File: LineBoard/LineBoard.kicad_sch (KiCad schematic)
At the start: 0 parts

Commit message: サイドセンサプルアップ追加
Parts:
- added C1: C_Small, Capacitor_SMD:C_0603_1608Metric_Pad1.08x0.95mm_HandSolder, symbol Device:C_Small
- added D1: IR17-21C/TR8, LED_SMD:LED_0805_2012Metric, symbol Device:LED
- added D2: IR17-21C/TR8, Diode_SMD:D_0805_2012Metric_Pad1.15x1.40mm_HandSolder, symbol Device:LED_Small
- added IC1: S7136, S7136:DIP575W60P254L560H210Q4N, symbol 0_Aslan2:S7136
- added J1: side_l, Connector_JST:JST_PH_B3B-PH-K_1x03_P2.00mm_Vertical, symbol Connector_Generic:Conn_01x03
- added Q1: PT17-21B/L41/TR8, Diode_SMD:D_0805_2012Metric, symbol Device:Q_Photo_NPN
- added R1: 180, Resistor_SMD:R_0603_1608Metric, symbol Device:R
- added R2: 10k, Resistor_SMD:R_0603_1608Metric, symbol Device:R
- added R3: 420, Resistor_SMD:R_0603_1608Metric_Pad0.98x0.95mm_HandSolder, symbol Device:R_Small
- added R4: 5.6k, Resistor_SMD:R_0402_1005Metric, symbol Device:R_Small
- added R5: 10k, Resistor_SMD:R_0402_1005Metric, symbol Device:R_Small
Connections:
- new net: D2.2 (A), R3.1
- new net: IC1.3 (VOUT), J1.3 (Pin_3), R4.2, R5.1
- new net: D2.1 (K), IC1.1 (CATHODE_(LED))
- new net: D1.2 (A), R1.2
- new net +3V3: Q1.1 (C)
- new net +5V: C1.1, IC1.2 (VCC), J1.2 (Pin_2), R1.1, R3.2, R4.1
- new net GND: C1.2, D1.1 (K), IC1.4 (GND), J1.1 (Pin_1), R2.2, R5.2
- new net VOUT: Q1.2 (E), R2.1
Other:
- note added: "IR17-21C/TR8 (5V) + PT17-21B/L41/TR8 (3.3V) reflective photo-reflector R1=180R sets IF≈21mA. R2=10k pull-up (tune experimentally by reflectance)."

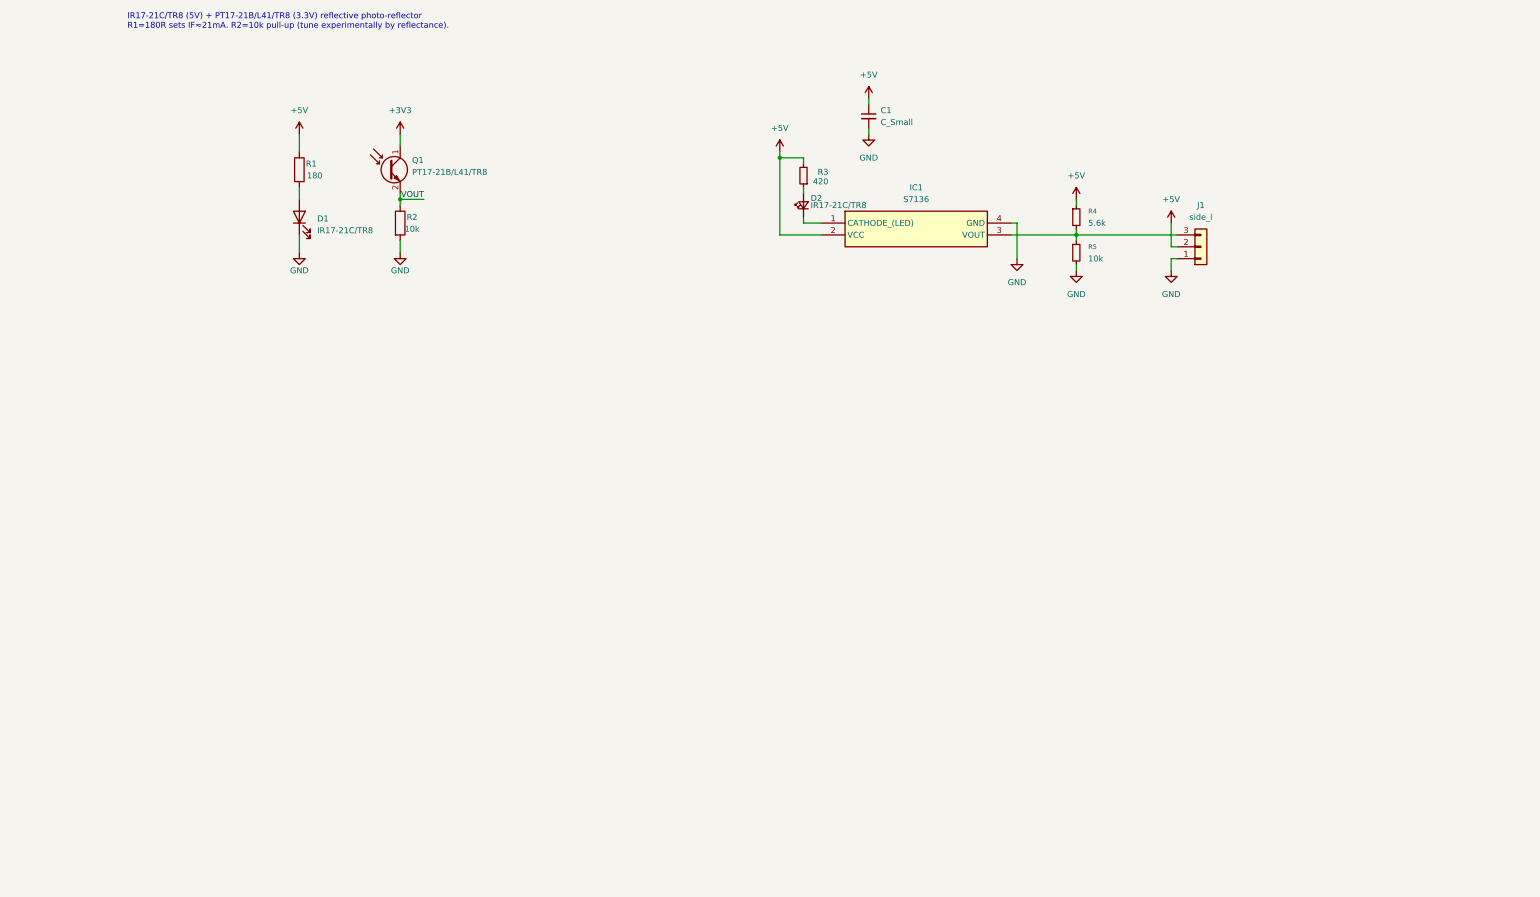
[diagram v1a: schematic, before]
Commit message: メイン基板完成
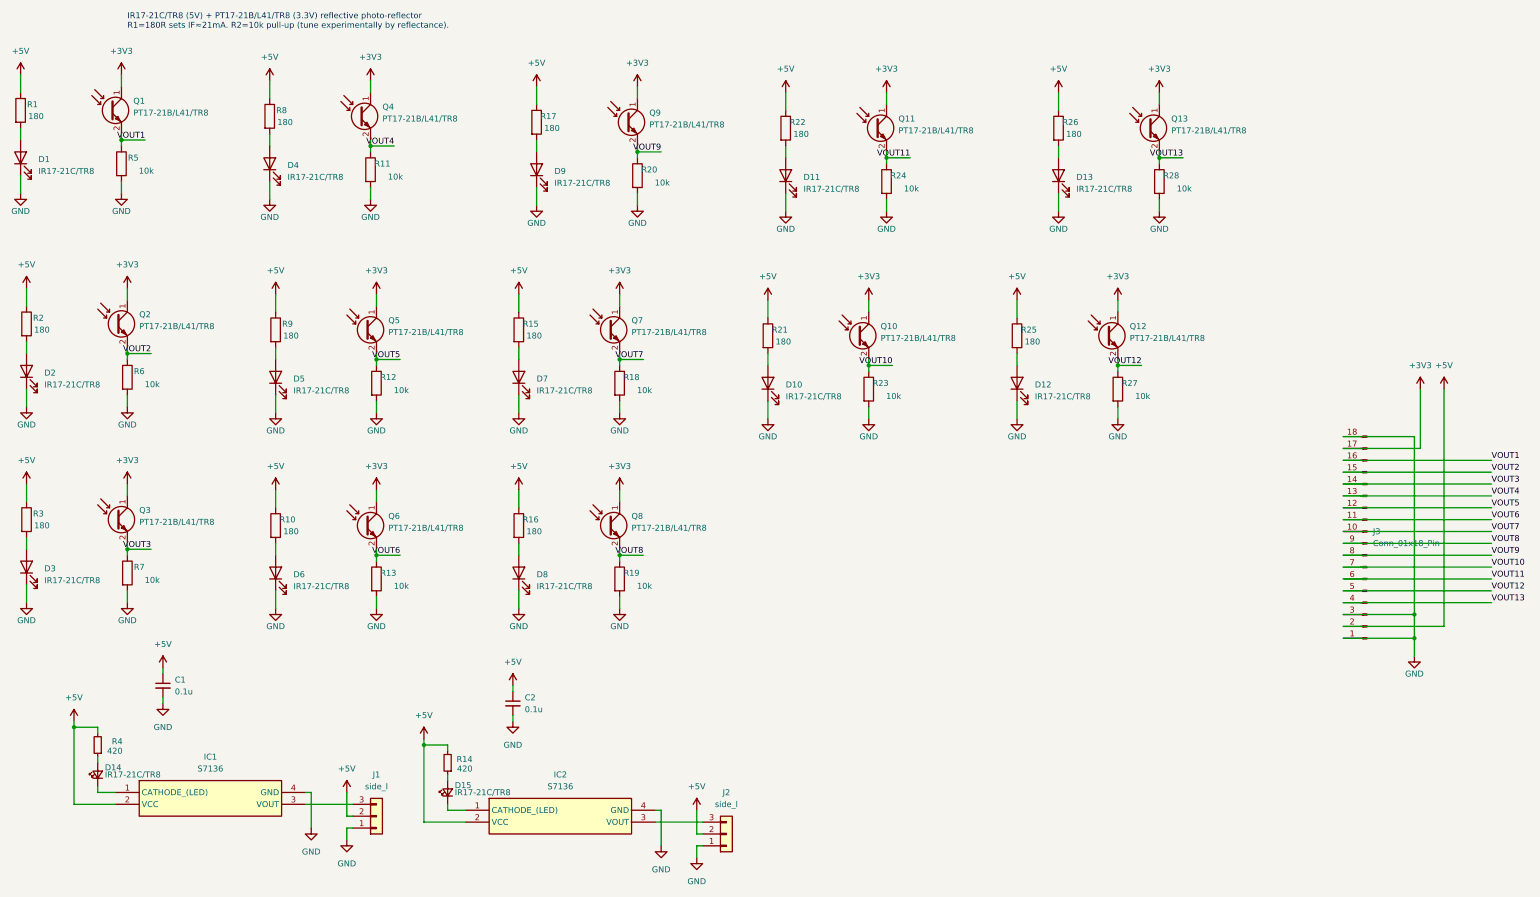
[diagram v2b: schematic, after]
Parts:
- removed R5: 10k, Resistor_SMD:R_0402_1005Metric, symbol Device:R_Small
- added C1: 0.1u, Capacitor_SMD:C_0603_1608Metric_Pad1.08x0.95mm_HandSolder, symbol Device:C_Small
- added D10, D11, D12, D13, D2, D3, D4, D5, D6, D7, D8, D9: IR17-21C/TR8, LED_SMD:LED_0805_2012Metric, symbol Device:LED
- added D14: IR17-21C/TR8, Diode_SMD:D_0805_2012Metric_Pad1.15x1.40mm_HandSolder, symbol Device:LED_Small
- added IC1: S7136, S7136:DIP575W60P254L560H210Q4N, symbol 0_Aslan2:S7136
- added J1: side_l, Connector_JST:JST_SH_BM03B-SRSS-TB_1x03-1MP_P1.00mm_Vertical, symbol Connector_Generic:Conn_01x03
- added J3: Conn_01x18_Pin, 5051101892:CON_5051101892_MOL, symbol Connector:Conn_01x18_Pin
- added Q10, Q11, Q12, Q13, Q2, Q3, Q4, Q5, Q6, Q7, Q8, Q9: PT17-21B/L41/TR8, Diode_SMD:D_0805_2012Metric, symbol Device:Q_Photo_NPN
- added R10, R15, R16, R17, R2, R21, R22, R25, R26, R3, R8, R9: 180, Resistor_SMD:R_0603_1608Metric, symbol Device:R
- added R11, R12, R13, R18, R19, R20, R23, R24, R27, R28, R6, R7: 10k, Resistor_SMD:R_0603_1608Metric, symbol Device:R
- C2: renamed from C1; value C_Small -> 0.1u
- J2: renamed from J1; footprint Connector_JST:JST_PH_B3B-PH-K_1x03_P2.00mm_Vertical -> Connector_JST:JST_SH_BM03B-SRSS-TB_1x03-1MP_P1.00mm_Vertical
- R14: renamed from R3; footprint Resistor_SMD:R_0603_1608Metric_Pad0.98x0.95mm_HandSolder -> Resistor_SMD:R_0603_1608Metric
- R4: value 5.6k -> 420; footprint Resistor_SMD:R_0402_1005Metric -> Resistor_SMD:R_0603_1608Metric
- renumbered D2 to D15, IC1 to IC2, R2 to R5
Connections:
- net +3V3: now also J3.17 (Pin_17), Q10.1 (C), Q11.1 (C), Q12.1 (C), Q13.1 (C), Q2.1 (C), Q3.1 (C), Q4.1 (C), Q5.1 (C), Q6.1 (C), Q7.1 (C), Q8.1 (C), Q9.1 (C)
- net +5V: now also R4.2, C1.1, IC1.2 (VCC), J1.2 (Pin_2), J3.2 (Pin_2), R10.1, R15.1, R16.1, R17.1, R2.1, R21.1, R22.1, R25.1, R26.1, R3.1, R8.1, R9.1; no longer R4.1
- net GND: now also C1.2, D10.1 (K), D11.1 (K), D12.1 (K), D13.1 (K), D2.1 (K), D3.1 (K), D4.1 (K), D5.1 (K), D6.1 (K), D7.1 (K), D8.1 (K), D9.1 (K), IC1.4 (GND), J1.1 (Pin_1), J3.1 (Pin_1), J3.18 (Pin_18), J3.3 (Pin_3), R11.2, R12.2, R13.2, R18.2, R19.2, R20.2, R23.2, R24.2, R27.2, R28.2, R6.2, R7.2
- net at IC2.3 (VOUT), J2.3 (Pin_3): no longer R4.2
- net VOUT renamed VOUT1
- net VOUT1: now also J3.16 (Pin_16)
- new net: D14.1 (K), IC1.1 (CATHODE_(LED))
- new net: IC1.3 (VOUT), J1.3 (Pin_3)
- new net: D2.2 (A), R2.2
- new net: D3.2 (A), R3.2
- new net: D13.2 (A), R26.2
- new net: D14.2 (A), R4.1
- new net: D6.2 (A), R10.2
- new net: D8.2 (A), R16.2
- new net: D4.2 (A), R8.2
- new net: D7.2 (A), R15.2
- new net: D9.2 (A), R17.2
- new net: D12.2 (A), R25.2
- new net: D5.2 (A), R9.2
- new net: D10.2 (A), R21.2
- new net: D11.2 (A), R22.2
- new net VOUT10: J3.7 (Pin_7), Q10.2 (E), R23.1
- new net VOUT11: J3.6 (Pin_6), Q11.2 (E), R24.1
- new net VOUT12: J3.5 (Pin_5), Q12.2 (E), R27.1
- new net VOUT13: J3.4 (Pin_4), Q13.2 (E), R28.1
- new net VOUT2: J3.15 (Pin_15), Q2.2 (E), R6.1
- new net VOUT3: J3.14 (Pin_14), Q3.2 (E), R7.1
- new net VOUT4: J3.13 (Pin_13), Q4.2 (E), R11.1
- new net VOUT5: J3.12 (Pin_12), Q5.2 (E), R12.1
- new net VOUT6: J3.11 (Pin_11), Q6.2 (E), R13.1
- new net VOUT7: J3.10 (Pin_10), Q7.2 (E), R18.1
- new net VOUT8: J3.9 (Pin_9), Q8.2 (E), R19.1
- new net VOUT9: J3.8 (Pin_8), Q9.2 (E), R20.1
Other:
- moved on the sheet: C2, D1, D15, IC2, J2, Q1, R1, R14, R5
